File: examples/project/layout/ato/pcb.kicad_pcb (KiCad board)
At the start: 2 copper layers, 2 parts

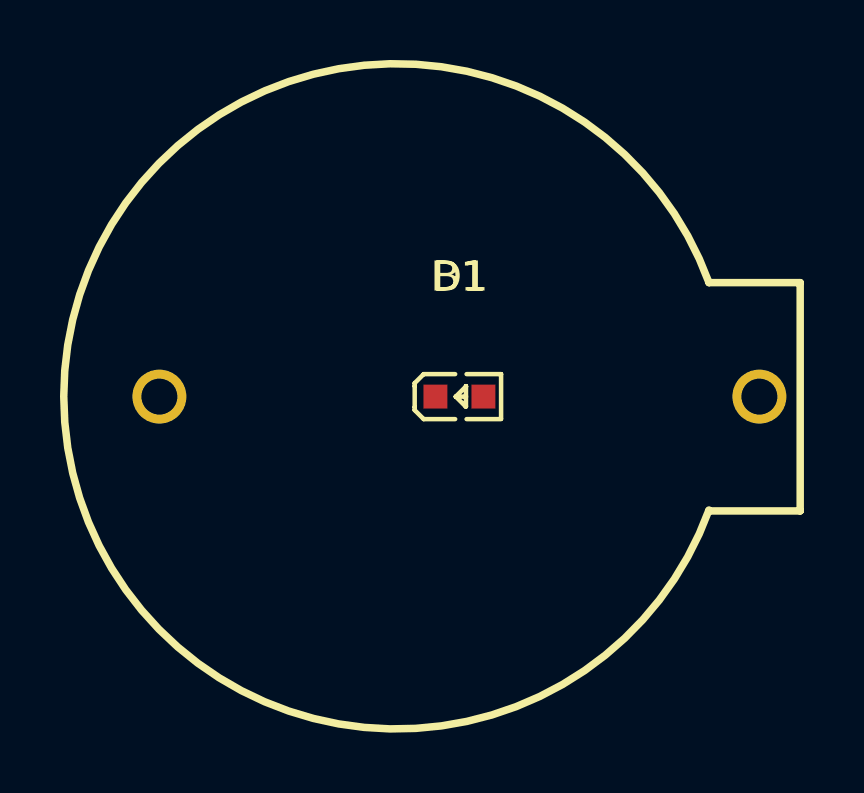
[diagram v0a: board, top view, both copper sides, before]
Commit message: CLI builds!
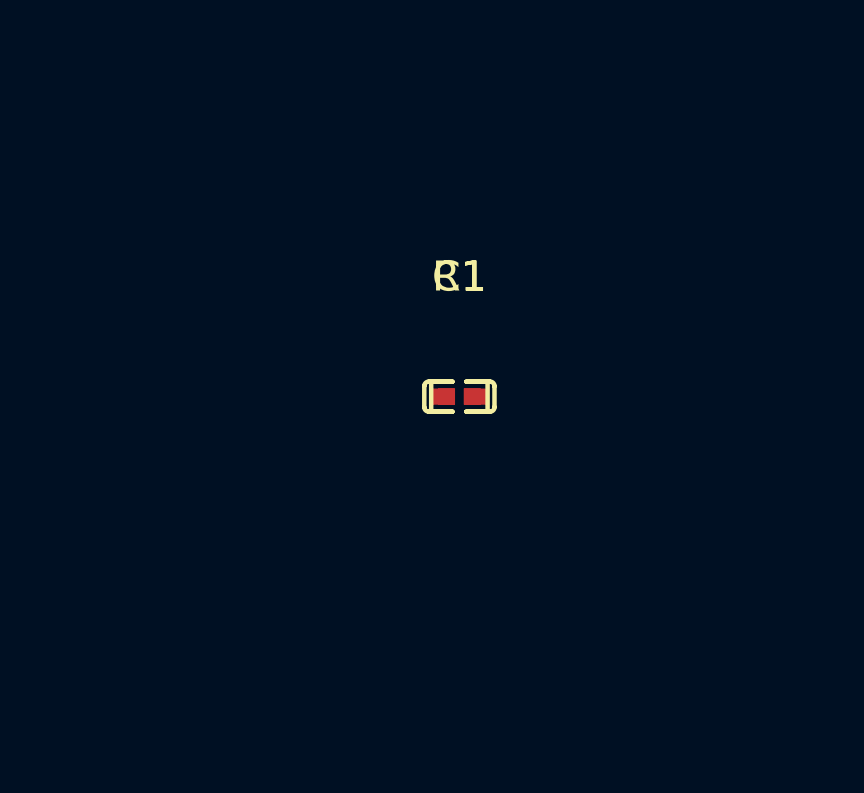
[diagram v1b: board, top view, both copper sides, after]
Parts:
- removed B1: Battery, lcsc:BAT-TH_BS-02-A1AJ010
- removed D1: PoweredLED, lcsc:LED0603-RD-YELLOW
- added C1: 100nF ±10% 16V X7R, lcsc:C0402, F.Cu at (0.00, 0.00)
- added R1: 10kΩ ±1% 62.5mW, lcsc:R0402, F.Cu at (0.00, 0.00)

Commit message: Exporters: Improve stability of netlist application
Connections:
- net *AA08-net-0 renamed net
- net *AA08-net-1 renamed net-1
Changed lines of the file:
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@@
             (outputdirectory "")))
     (net 0 "")
-    (net 2 "*AA08-net-1")
-    (net 3 "*AA08-net-0")
+    (net 2 "net-1")
+    (net 3 "net")
     (footprint "lcsc:R0402"
         (layer "F.Cu")
@@
             (layers "F.Cu" "F.Paste" "F.Mask")
             (remove_unused_layers no)
-            (net 2 "*AA08-net-1")
+            (net 2 "net-1")
 )
         (pad "1" smd rect
@@
             (layers "F.Cu" "F.Paste" "F.Mask")
             (remove_unused_layers no)
-            (net 3 "*AA08-net-0")
+            (net 3 "net")
 )
         (model "${KIPRJMOD}/../libs/3dmodels/lcsc.3dshapes/R0402_L1.0-W0.5-H0.5.wrl"
@@
             (layers "F.Cu" "F.Paste" "F.Mask")
             (remove_unused_layers no)
-            (net 2 "*AA08-net-1")
+            (net 2 "net-1")
 )
         (pad "1" smd rect
@@
             (layers "F.Cu" "F.Paste" "F.Mask")
             (remove_unused_layers no)
-            (net 3 "*AA08-net-0")
+            (net 3 "net")
 )
         (model "${KIPRJMOD}/../libs/3dmodels/lcsc.3dshapes/C0402_L1.0-W0.5-H0.5.wrl"
